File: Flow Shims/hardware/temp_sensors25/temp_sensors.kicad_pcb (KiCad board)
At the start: 2 copper layers, 6 x 113 mm, 52 parts, among them J1 Conn_01x03, U10 TMP1826NG, U11 TMP1826NG, U12 TMP1826NG, U13 TMP1826NG, U14 TMP1826NG, U15 TMP1826NG, U16 TMP1826NG, U17 TMP1826NG, U18 TMP1826NG, U19 TMP1826NG, U2 TMP1826NG, U20 TMP1826NG, U21 TMP1826NG, U22 TMP1826NG, U23 TMP1826NG, U24 TMP1826NG, U25 TMP1826NG, U26 TMP1826NG, U3 TMP1826NG, U4 TMP1826NG, U5 TMP1826NG, U6 TMP1826NG, U7 TMP1826NG, U8 TMP1826NG, U9 TMP1826NG

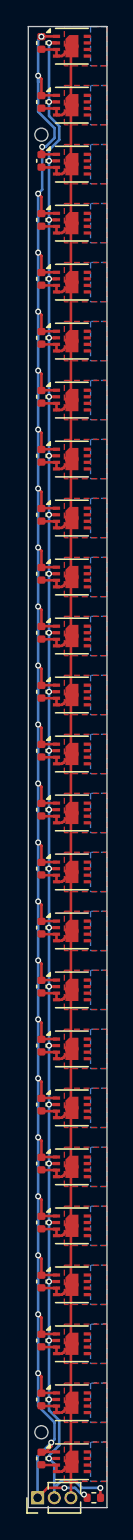
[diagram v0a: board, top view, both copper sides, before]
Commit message: All boards DRC/ERC clean
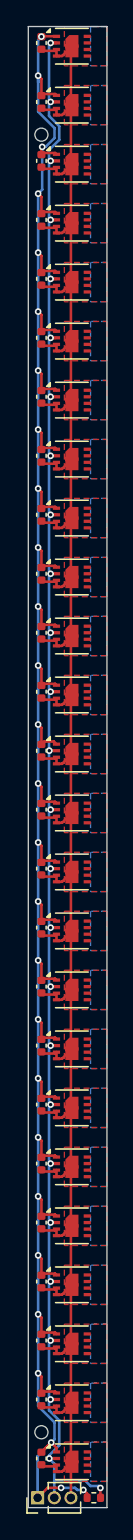
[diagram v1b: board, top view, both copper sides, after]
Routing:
- net +3.3V: track 184.6 -> 187.4 mm
- net GND: track 187.8 -> 190.0 mm
